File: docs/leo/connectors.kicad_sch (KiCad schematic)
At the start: 9 parts, among them CN1_A Conn_01x32, CN1_B Conn_01x32, CN1_C Conn_01x32, CN2_A Conn_01x32, CN2_B Conn_01x32, CN2_C Conn_01x32, CN3_A Conn_01x32, CN3_B Conn_01x32

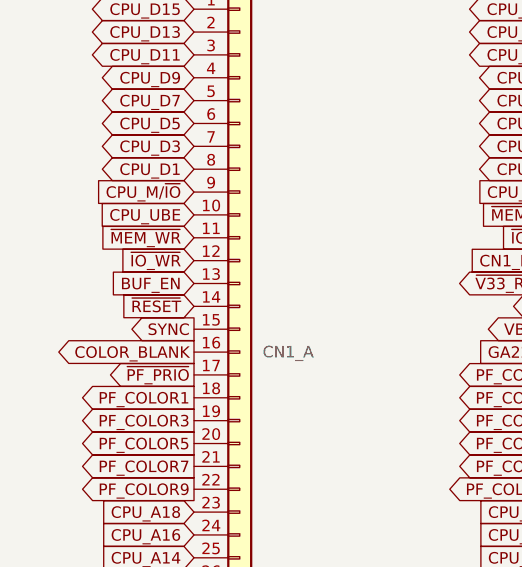
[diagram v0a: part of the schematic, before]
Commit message: Add more b board logic
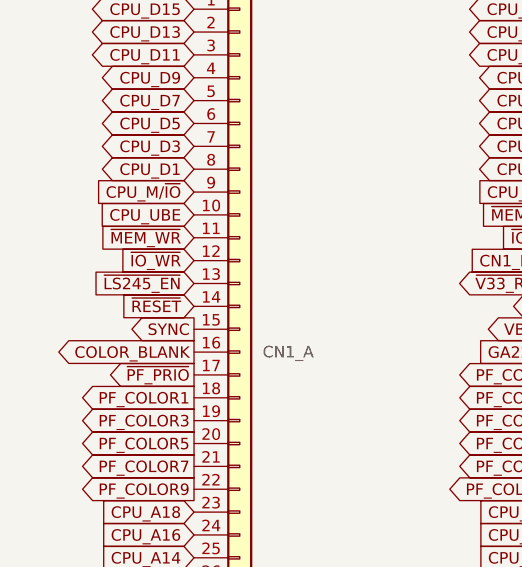
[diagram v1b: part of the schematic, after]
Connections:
- net BUF_EN renamed ~{LS245_EN}
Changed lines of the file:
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@@
     )
   )
-  (global_label "BUF_EN" (shape input) (at 35.56 49.53 180) (fields_autoplaced)
+  (global_label "~{LS245_EN}" (shape input) (at 35.56 49.53 180) (fields_autoplaced)
     (effects (font (size 1.27 1.27)) (justify right))
     (property "Intersheet References" "${INTERSHEET_REFS}" (id 0) (at 25.1036 49.4506 0)
